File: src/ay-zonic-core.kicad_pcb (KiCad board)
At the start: 2 copper layers, 61 x 80.6 mm, 31 parts, among them SW1 ZON-X, U1 AY-3-8912, U2 74HCT74, U3 74HCT08, U4 74HCT11, U5 74HCT02

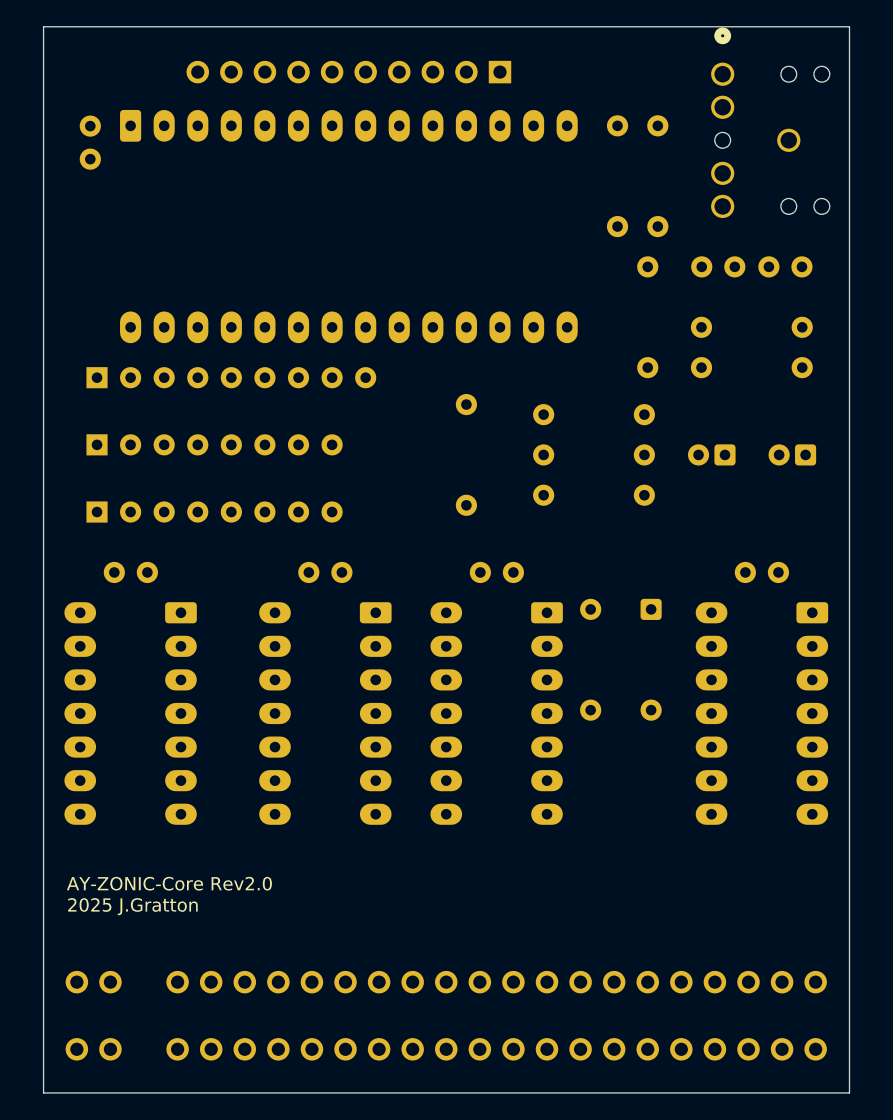
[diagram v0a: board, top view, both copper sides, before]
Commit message: routed and new images
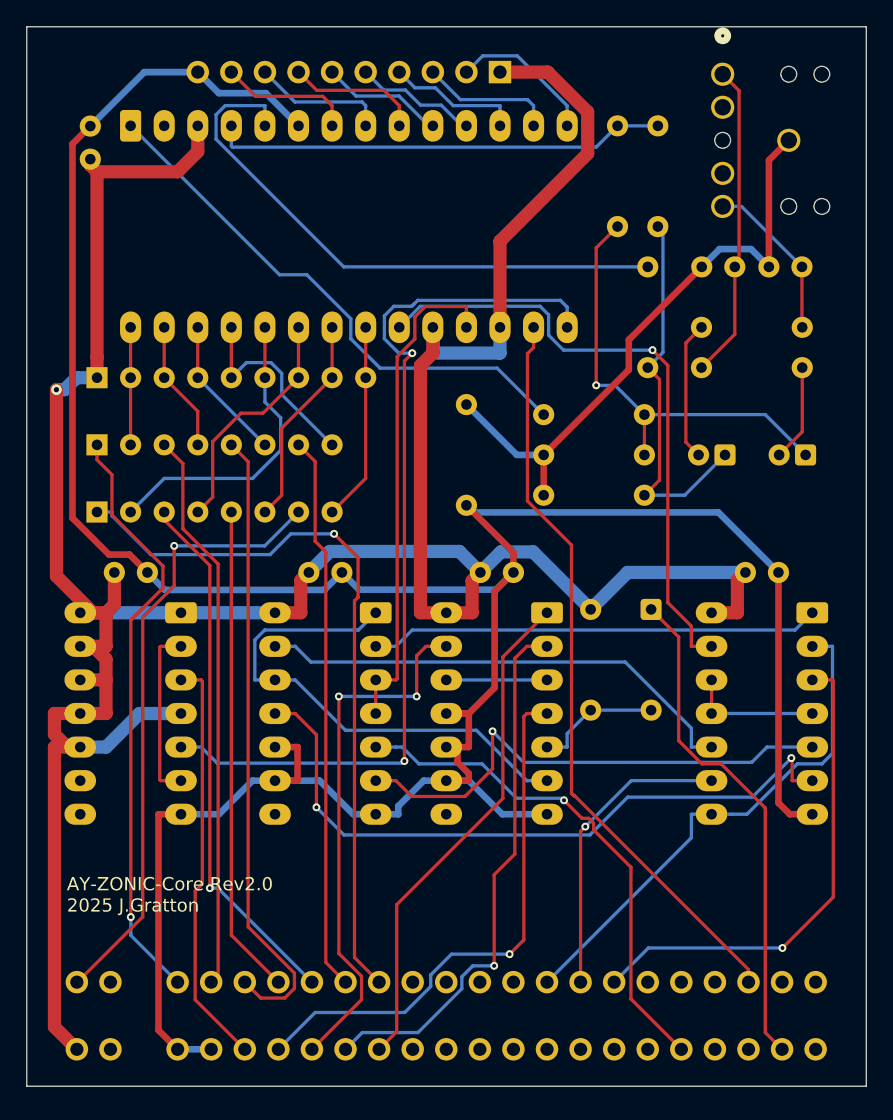
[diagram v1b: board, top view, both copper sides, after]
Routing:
- net VCC: track 0.00 -> 234.9 mm, vias 0 -> 1
- net GND: track 0.00 -> 224.3 mm
- net /PSGCLK: track 0.00 -> 69.2 mm, vias 0 -> 2
- net /~{RESET}: track 0.00 -> 56.9 mm
- net /D4: track 0.00 -> 55.6 mm, vias 0 -> 1
- net Net-(U3-Pad11): track 0.00 -> 51.7 mm, vias 0 -> 2
- net /D2: track 0.00 -> 47.6 mm
- net /BC1: track 0.00 -> 47.2 mm, vias 0 -> 1
- net /D7: track 0.00 -> 46.5 mm, vias 0 -> 1
- net GND_AUDIO: track 0.00 -> 46.0 mm
- net /D0: track 0.00 -> 45.2 mm, vias 0 -> 1
- net /OUTA: track 0.00 -> 44.0 mm
- net /D1: track 0.00 -> 42.5 mm
- net /D3: track 0.00 -> 42.1 mm
- net /A0: track 0.00 -> 41.3 mm, vias 0 -> 1
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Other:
- board size 61 x 80.6 mm -> 63.5 x 80.1 mm
